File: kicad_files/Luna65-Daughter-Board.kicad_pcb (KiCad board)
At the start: 2 copper layers, 25.1 x 25.1 mm, 38 parts, among them J1 TYPE-C-31-M12, J2 Molex Power, J3 JSTPH, Q1 MMUN2133LT1G, U1 MCP73831, U2 USBLC6-2SC6, U3 AP2112, U4 APX803L, U5 TPS61032RSAR

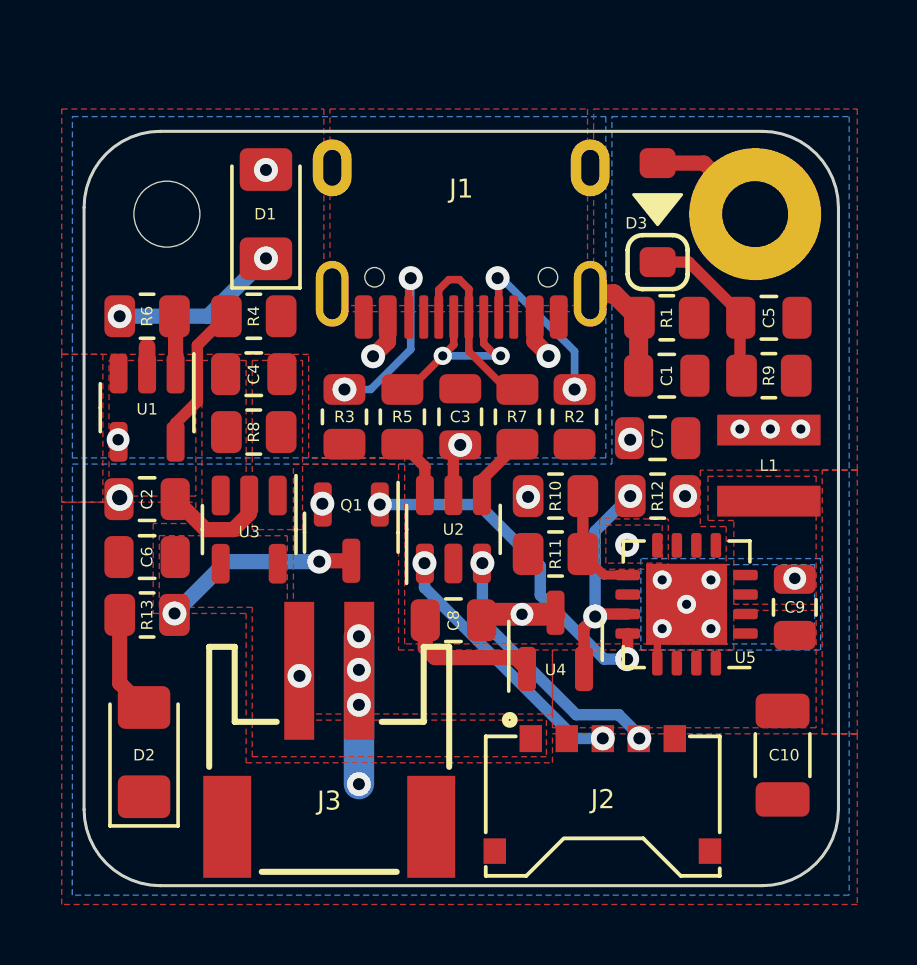
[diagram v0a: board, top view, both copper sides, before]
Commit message: DB Rev 4 Changes
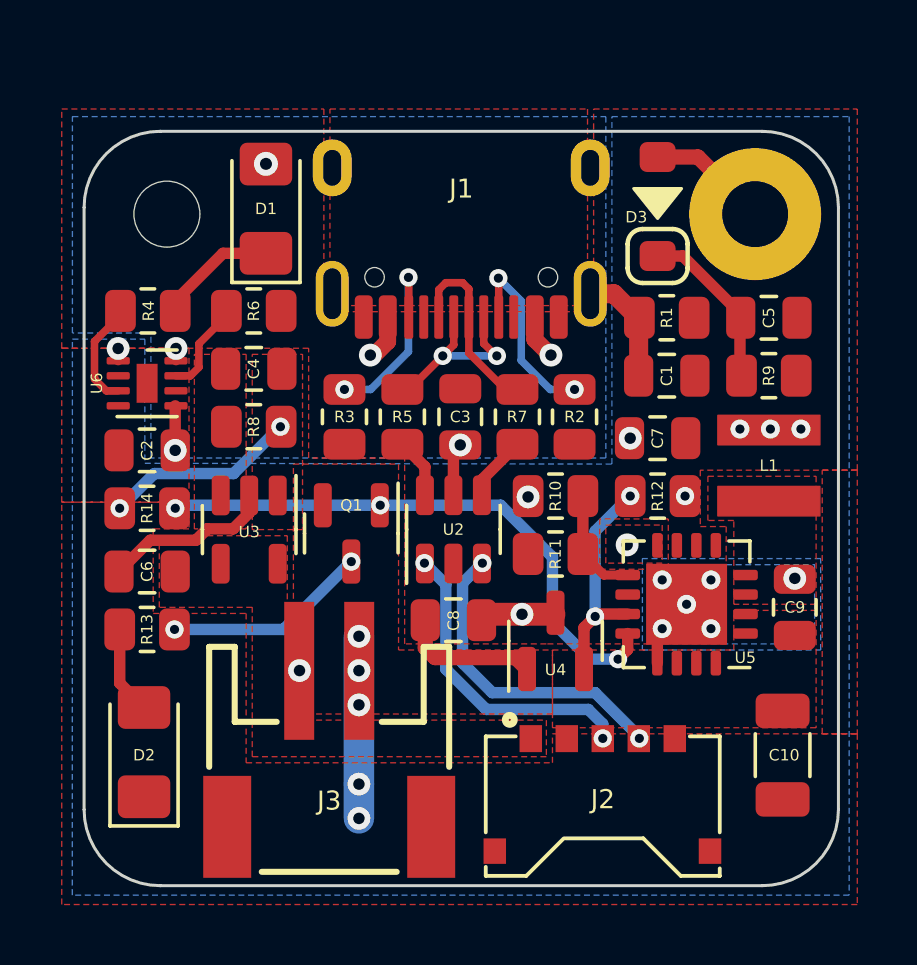
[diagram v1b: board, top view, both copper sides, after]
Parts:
- removed U1: MCP73831, Package_TO_SOT_SMD:SOT-23-5
- added R14: 1K, Resistor_SMD:R_0805_2012Metric, F.Cu at (92.3, 62.5)
- added U6: LTC4095, Package_DFN_QFN:DFN-8-1EP_2x2mm_P0.5mm_EP0.7x1.3mm, F.Cu at (92.3, 58.3)
- C2: value 10uF -> 1uF
- Q1: value MMUN2133LT1G -> TP0610T
- R4: value 2K -> 1K
- R6: value 1K -> 842
- moved R6 3.56 mm to (95.9, 55.9), turned to 0 degrees
- moved R4 3.54 mm to (92.4, 55.9)
- moved C2 1.63 mm to (92.3, 60.5)
- moved C6 0.48 mm to (92.3, 64.6)
- moved R13 0.48 mm to (92.3, 66.5)
- moved D3 0.20 mm to (109.3, 52.4)
- moved D1 0.18 mm to (96.3, 52.5)
- moved C4 0.18 mm to (95.9, 57.8)
- moved R8 0.18 mm to (95.9, 59.7)
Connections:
- C2 pad 1: GND -> VUSB
- C2 pad 2: VBAT -> GND
- Q1 pad 2: VBAT -> 5V
- R4 pad 2: GND -> Net-(D1-Pad1)
- R6 pad 2: Net-(D1-Pad1) -> GND
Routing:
- net /LBO: track 11.8 -> 19.2 mm, vias 2 -> 3
- net 5V: track 0.00 -> 6.49 mm, vias 0 -> 2
- net GND: track 15.1 -> 17.4 mm, vias 10 -> 11
- net Net-(D1-Pad1): track 5.68 -> 3.72 mm, vias 2 -> 0
- net VUSB: track 4.45 -> 6.35 mm, vias 5 -> 6
- net D+: track 8.84 -> 10.6 mm
- net D-: track 8.84 -> 10.3 mm
- net Net-(R4-Pad1): track 4.84 -> 3.39 mm
- net Net-(R6-Pad1): track 1.82 -> 2.96 mm
- net Net-(D2-Pad2): track 3.52 -> 2.94 mm
- net VBAT: track 2.50 -> 2.91 mm, vias 11 -> 10

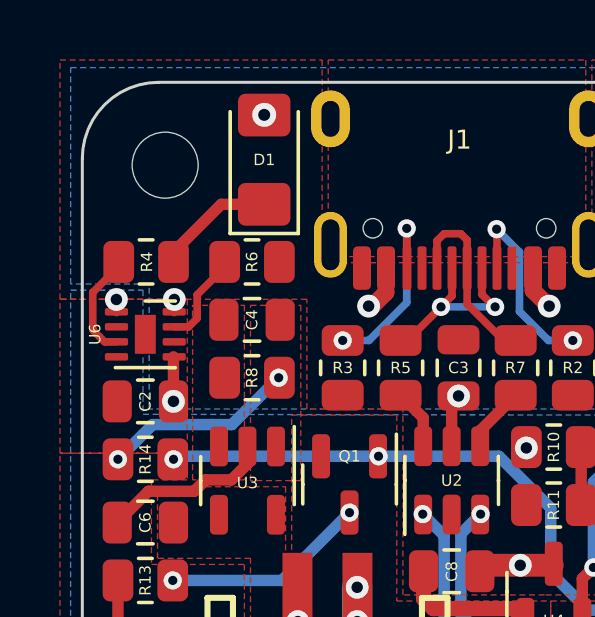
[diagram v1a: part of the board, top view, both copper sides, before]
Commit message: V7 Changes
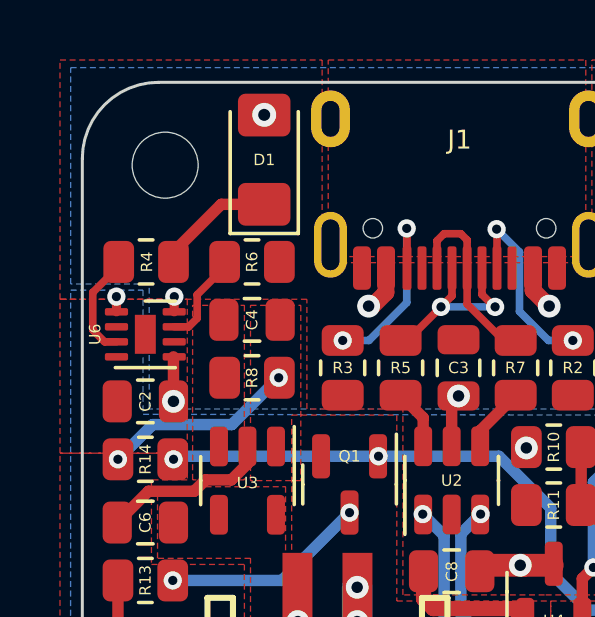
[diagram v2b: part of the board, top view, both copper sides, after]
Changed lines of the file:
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@@
   (segment (start 105.791 57.3532) (end 105.772794 57.3532) (width 0.5588) (layer "F.Cu") (net 4))
   (segment (start 105.772794 57.3532) (end 105.251141 56.831547) (width 0.5588) (layer "F.Cu") (net 4))
+  (segment (start 93.2915 57.0394) (end 93.2915 57.543) (width 0.3048) (layer "F.Cu") (net 4))
   (segment (start 100.351141 56.898864) (end 100.351141 56.084437) (width 0.5588) (layer "F.Cu") (net 4))
+  (segment (start 93.2942 57.0367) (end 93.2915 57.0394) (width 0.3048) (layer "F.Cu") (net 4))
   (segment (start 93.2661 59.043) (end 93.2661 60.5278) (width 0.381) (layer "F.Cu") (net 4))
   (segment (start 99.861364 57.388641) (end 100.351141 56.898864) (width 0.5588) (layer "F.Cu") (net 4))
-  (segment (start 93.2942 57.1319) (end 93.2915 57.1346) (width 0.3048) (layer "F.Cu") (net 4))
   (segment (start 102.5398 62.0245) (end 102.5398 60.5767) (width 0.381) (layer "F.Cu") (net 4))
-  (segment (start 93.2915 57.1346) (end 93.2915 57.543) (width 0.3048) (layer "F.Cu") (net 4))
   (via (at 96.2914 50.9778) (size 0.8) (drill 0.4) (layers "F.Cu" "B.Cu") (net 4))
-  (via (at 93.2942 57.13189) (size 0.762) (drill 0.381) (layers "F.Cu" "B.Cu") (net 4))
+  (via (at 93.2942 57.0367) (size 0.6096) (drill 0.3048) (layers "F.Cu" "B.Cu") (net 4))
   (via (at 93.266108 60.527794) (size 0.762) (drill 0.381) (layers "F.Cu" "B.Cu") (net 4))
   (via (at 99.7712 57.3532) (size 0.762) (drill 0.381) (layers "F.Cu" "B.Cu") (net 4))
@@
   (segment (start 102.8446 64.9478) (end 103.505 64.2874) (width 0.381) (layer "B.Cu") (net 18))
   (segment (start 104.9274 65.9915) (end 105.8926 65.9915) (width 0.762) (layer "F.Cu") (net 20))
+  (segment (start 91.3665 57.0394) (end 91.3665 57.543) (width 0.3048) (layer "F.Cu") (net 20))
+  (segment (start 91.3638 57.0367) (end 91.3665 57.0394) (width 0.3048) (layer "F.Cu") (net 20))
   (segment (start 103.6759 65.9915) (end 103.4773 66.1901) (width 0.762) (layer "F.Cu") (net 20))
   (segment (start 104.9274 65.9915) (end 103.6759 65.9915) (width 0.762) (layer "F.Cu") (net 20))
-  (segment (start 91.3638 57.1319) (end 91.3665 57.1346) (width 0.3048) (layer "F.Cu") (net 20))
-  (segment (start 91.3665 57.1346) (end 91.3665 57.543) (width 0.3048) (layer "F.Cu") (net 20))
-  (via (at 91.3638 57.13189) (size 0.762) (drill 0.381) (layers "F.Cu" "B.Cu") (net 20))
+  (via (at 91.3638 57.0367) (size 0.6096) (drill 0.3048) (layers "F.Cu" "B.Cu") (net 20))
   (via (at 112.0902 59.817) (size 0.635) (drill 0.3048) (layers "F.Cu" "B.Cu") (net 20))
   (via (at 110.2614 62.0522) (size 0.6096) (drill 0.3048) (layers "F.Cu" "B.Cu") (net 20))

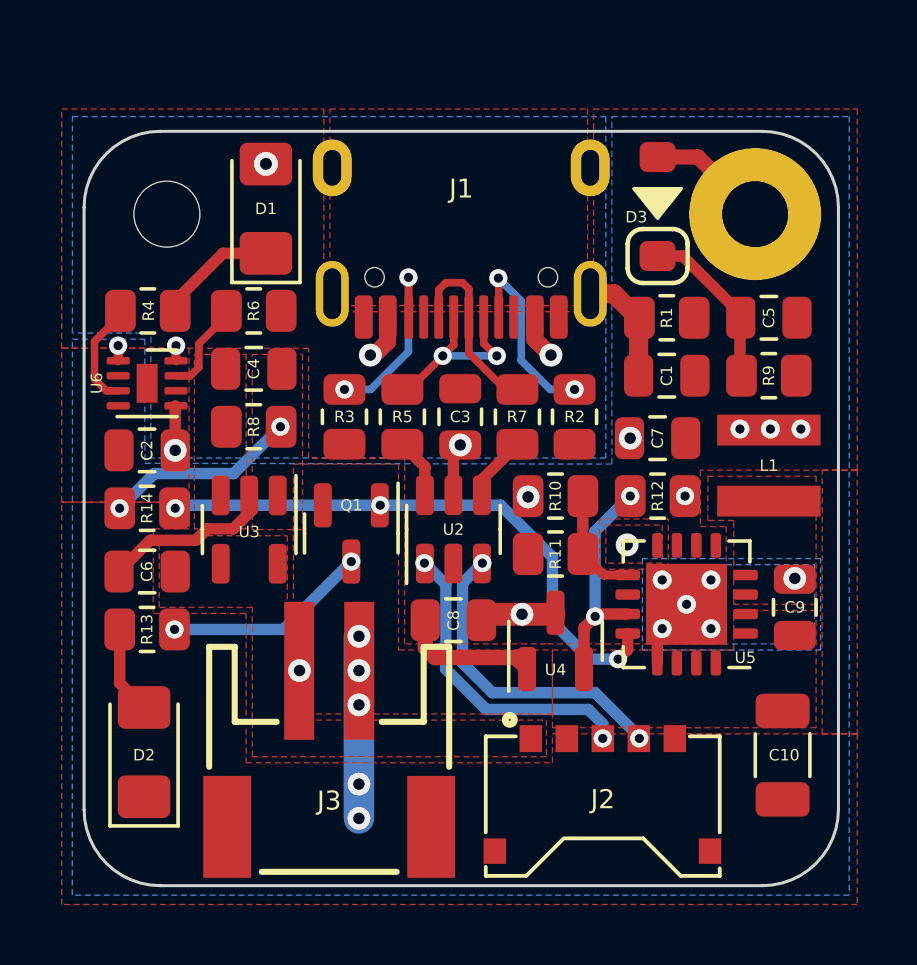
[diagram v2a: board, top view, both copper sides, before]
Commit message: stuff
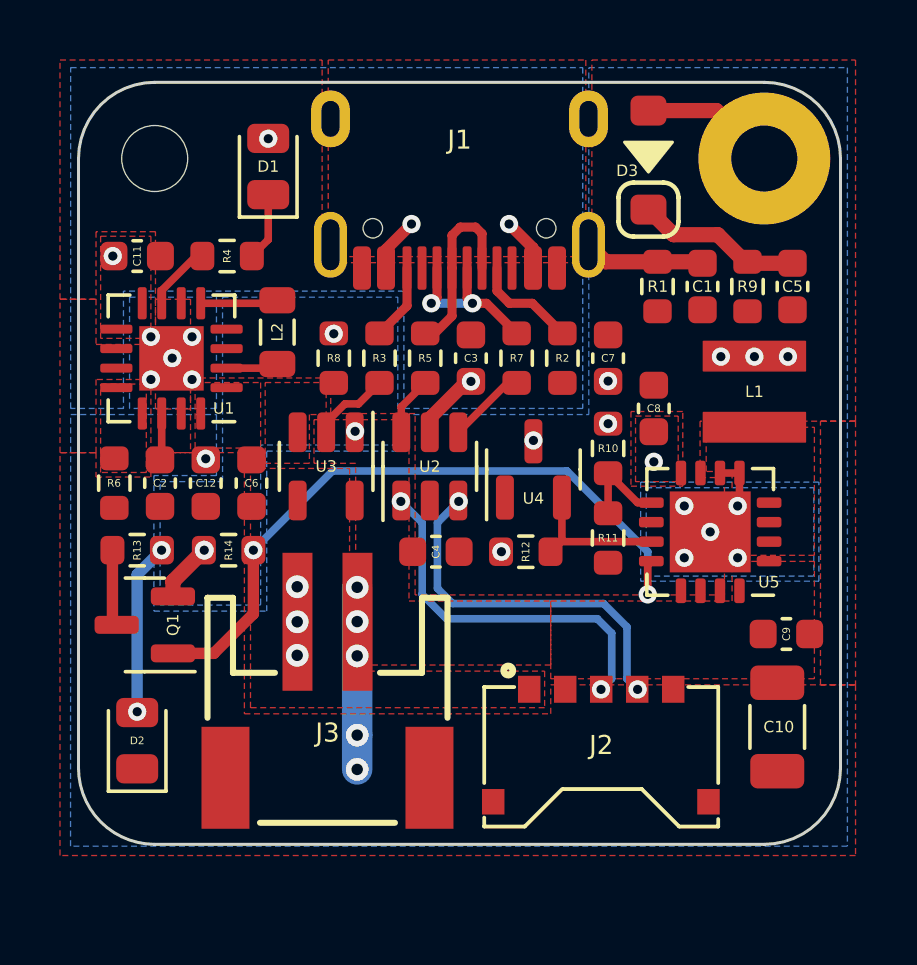
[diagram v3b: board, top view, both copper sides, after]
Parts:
- removed U6: LTC4095, Package_DFN_QFN:DFN-8-1EP_2x2mm_P0.5mm_EP0.7x1.3mm
- added C11: 10uF, Capacitor_SMD:C_0603_1608Metric, F.Cu at (92.0, 54.1)
- added C12: 10uF, Capacitor_SMD:C_0603_1608Metric, F.Cu at (94.3, 61.6)
- added L2: 1.5uH, Inductor_SMD:L_0805_2012Metric, F.Cu at (96.7, 56.6)
- added U1: LTC4001, Package_DFN_QFN:QFN-16-1EP_4x4mm_P0.65mm_EP2.15x2.15mm, F.Cu at (93.1, 57.5)
- C1, C3, C4, C5, C6, C7, C8, C9: footprint acheron_Components:C_0805_2012Metric -> Capacitor_SMD:C_0603_1608Metric
- C2: value 1uF -> 0.1uF; footprint acheron_Components:C_0805_2012Metric -> Capacitor_SMD:C_0603_1608Metric
- D1, D2: footprint LED_SMD:LED_1206_3216Metric_Pad1.42x1.75mm_HandSolder -> LED_SMD:LED_0805_2012Metric
- R1, R10, R11, R12, R13, R14, R2, R3, R4, R5, R7, R8, R9: footprint Resistor_SMD:R_0805_2012Metric -> Resistor_SMD:R_0603_1608Metric
- R6: value 842 -> 274; footprint Resistor_SMD:R_0805_2012Metric -> Resistor_SMD:R_0603_1608Metric
- moved C8 9.72 mm to (109.2, 59.1), turned to 90 degrees
- moved C4 8.60 mm to (102.0, 63.9), turned to 0 degrees
- moved Q1 7.53 mm to (92.3, 66.3), turned to 180 degrees
- moved R6 7.39 mm to (91.2, 61.6), turned to 90 degrees
- moved U4 5.76 mm to (105.2, 61.2)
- moved R12 4.77 mm to (105.0, 63.9), turned to 0 degrees
- moved C6 4.56 mm to (95.8, 61.6), turned to 90 degrees
- moved R8 3.51 mm to (98.6, 57.5), turned to -90 degrees
- moved U3 3.32 mm to (98.3, 61.1)
- moved R4 3.21 mm to (95.0, 54.1)
- moved C1 3.20 mm to (110.8, 55.1), turned to 90 degrees
- moved C7 3.14 mm to (107.7, 57.5), turned to 90 degrees
- moved R9 3.06 mm to (112.3, 55.1), turned to 90 degrees
- moved R14 3.06 mm to (95.0, 63.9)
- moved R13 2.66 mm to (92.0, 63.9), turned to 0 degrees
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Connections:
- C2 pad 1: VUSB -> Net-(C2-Pad1)
- R6 pad 1: Net-(R6-Pad1) -> GND
- R6 pad 2: GND -> Net-(R6-Pad2)
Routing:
- net GND: track 17.4 -> 10.1 mm, vias 11 -> 15
- net 5V: track 6.49 -> 1.97 mm, vias 2 -> 3
- net Net-(Q1-Pad3): track 6.83 -> 2.35 mm, vias 2 -> 0
- net /LBO: track 19.2 -> 23.3 mm, vias 3 -> 2
- net Net-(J1-PadB5): track 6.46 -> 2.56 mm, vias 2 -> 0
- net Net-(J1-PadA5): track 6.54 -> 3.53 mm, vias 2 -> 0
- net VBAT: track 3.00 -> 0.00 mm, vias 10 -> 12
- net Net-(R6-Pad1): track 2.96 -> 0.00 mm
- net Net-(D2-Pad2): track 2.94 -> 5.72 mm, vias 0 -> 2
- net Net-(L2-Pad1): track 0.00 -> 2.45 mm
- net /EN: track 7.52 -> 5.46 mm, vias 2 -> 0
- net D-: track 10.3 -> 12.3 mm
- net D+: track 10.6 -> 12.3 mm
- net Net-(L2-Pad2): track 0.00 -> 1.55 mm
- net Net-(C2-Pad1): track 0.00 -> 1.49 mm
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- added copper zone on B.Cu, net 5V
- added copper zone on F.Cu, net Net-(R6-Pad2)
- added copper zone on F.Cu, net VUSB
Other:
- board size 25.1 x 25.1 mm -> 25.4 x 25.4 mm
